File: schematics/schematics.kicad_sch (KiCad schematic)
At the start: 14 parts, among them J1 Conn_01x06_Pin, Q1 BC547, Q2 BC547, Q3 SFH309, SW1 SW_DPDT_x2, U1 ATtiny414-SS

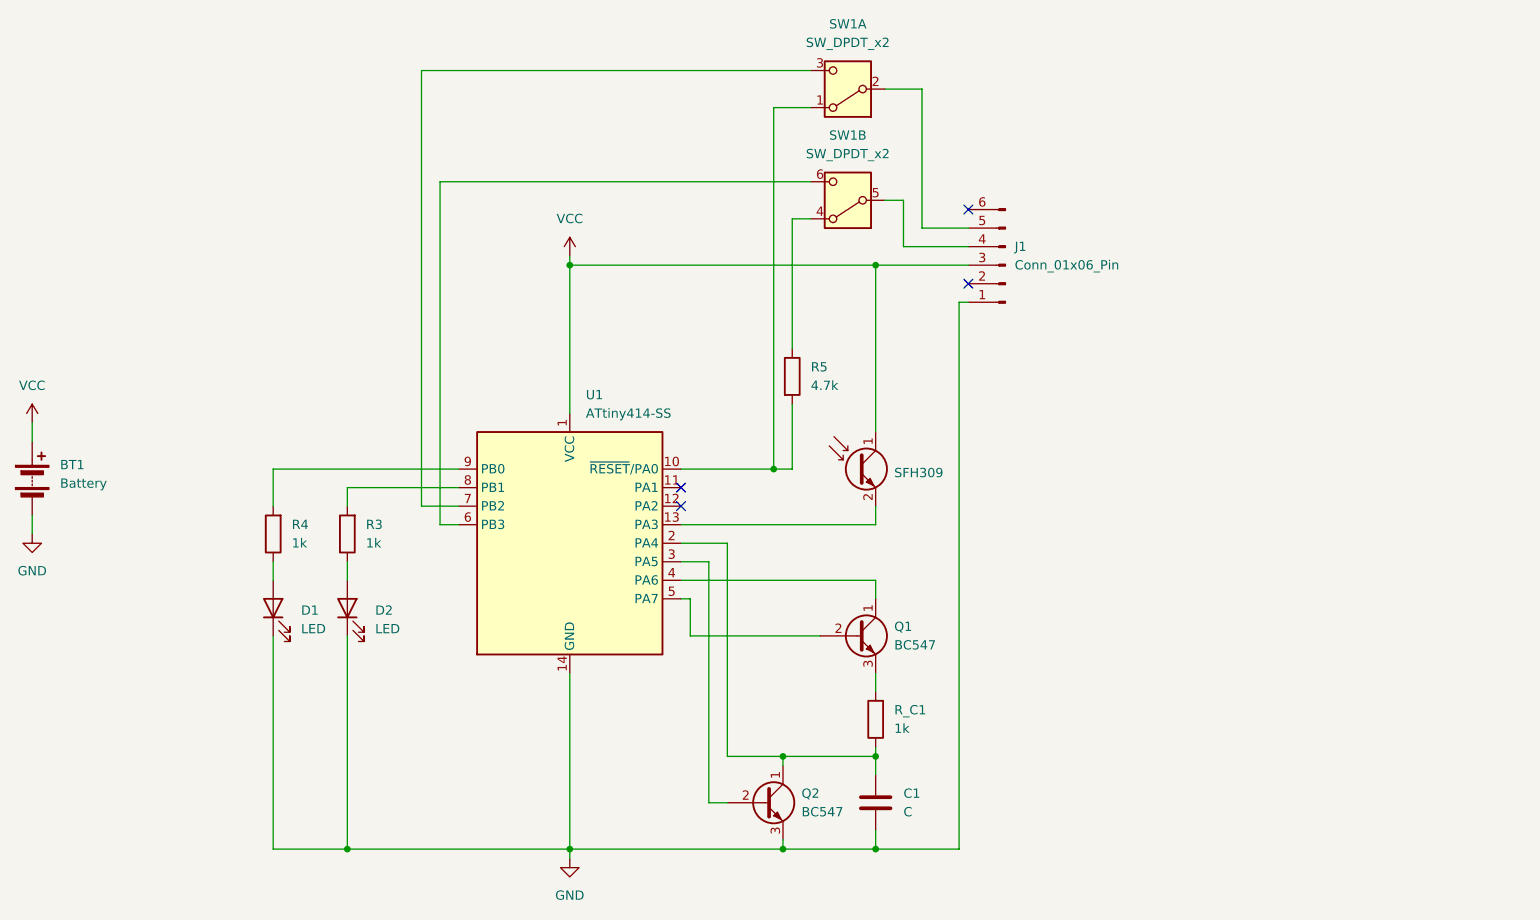
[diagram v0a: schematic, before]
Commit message: PCB ordered
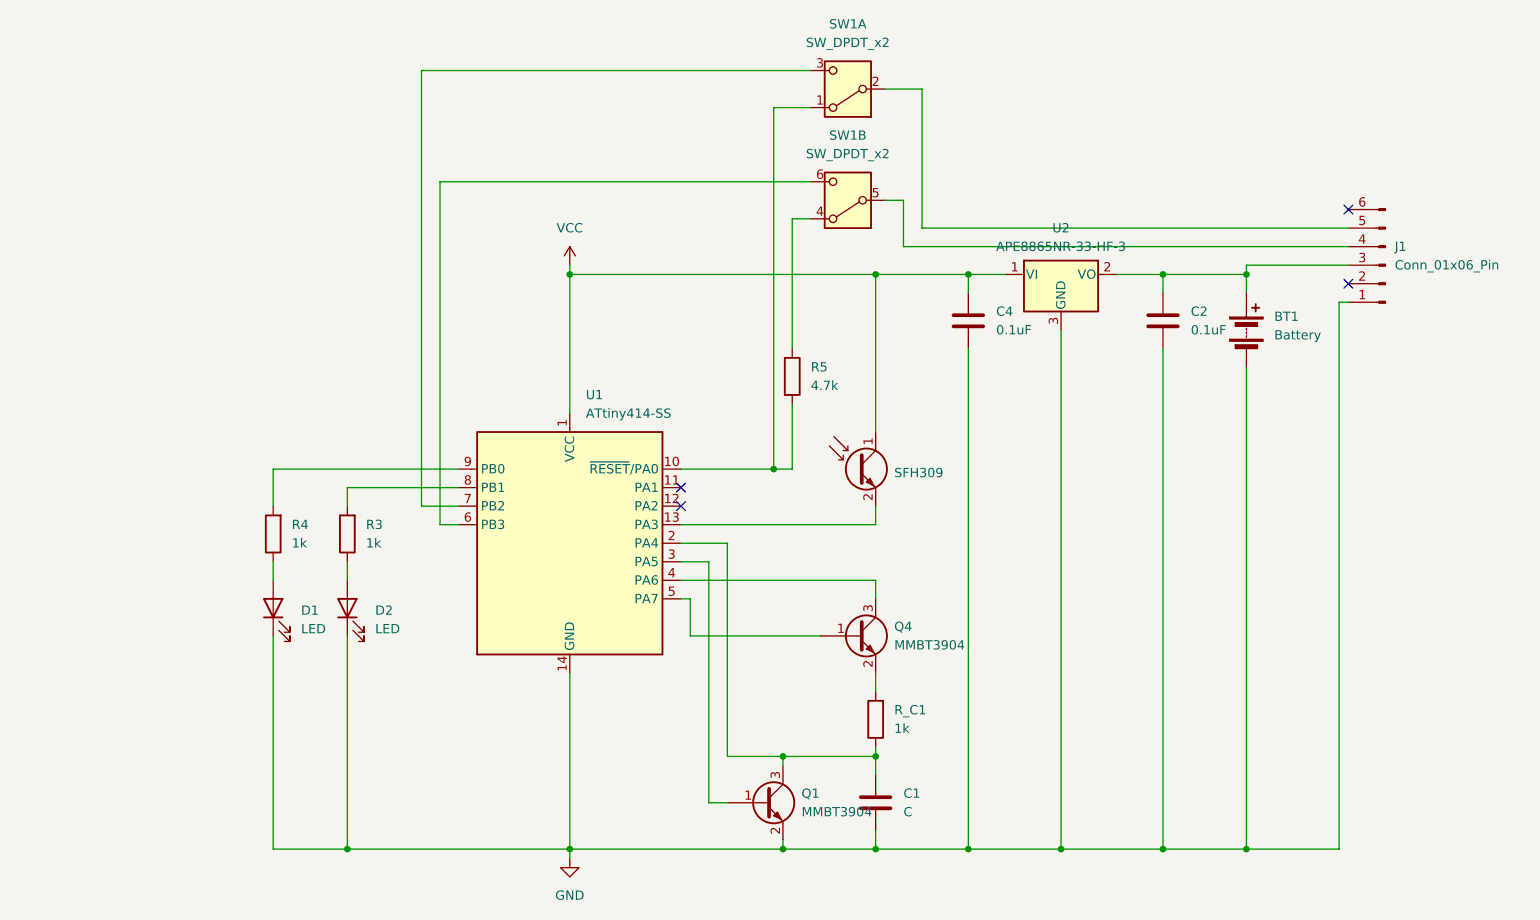
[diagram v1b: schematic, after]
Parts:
- removed Q1, Q2: BC547, Package_TO_SOT_THT:TO-92_Inline, symbol Transistor_BJT:BC547
- added C2, C4: 0.1uF, Capacitor_SMD:C_0805_2012Metric_Pad1.18x1.45mm_HandSolder, symbol Device:C
- added Q1, Q4: MMBT3904, Package_TO_SOT_SMD:SOT-23, symbol Transistor_BJT:MMBT3904
- added U2: APE8865NR-33-HF-3, Package_TO_SOT_SMD:SOT-23, symbol Regulator_Linear:APE8865NR-33-HF-3
- BT1: footprint Battery:BatteryHolder_Keystone_2479_3xAAA -> Battery:BatteryHolder_MPD_BH-18650-PC2
- R_C1: footprint Resistor_THT:R_Axial_DIN0207_L6.3mm_D2.5mm_P10.16mm_Horizontal -> Resistor_THT:R_Axial_DIN0207_L6.3mm_D2.5mm_P2.54mm_Vertical
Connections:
- net GND: now also C2.2, C4.2, Q1.2 (E), U2.3 (GND)
- net VCC: now also C4.1, U2.1 (VI); no longer BT1.1 (+), J1.3 (Pin_3)
- net at C1.1, R_C1.1, U1.2 (PA4): now also Q1.3 (C)
- net at U1.3 (PA5): now also Q1.1 (B)
- net at U1.4 (PA6): now also Q4.3 (C)
- net at U1.5 (PA7): now also Q4.1 (B)
- net at R_C1.2: now also Q4.2 (E)
- new net: BT1.1 (+), C2.1, J1.3 (Pin_3), U2.2 (VO)
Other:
- moved on the sheet: BT1, J1
